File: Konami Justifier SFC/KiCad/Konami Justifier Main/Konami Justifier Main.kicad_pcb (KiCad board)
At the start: 4 copper layers, 25.2 x 50 mm, 19 parts, among them J1 RJ12, J2 Conn_01x06_Socket, U1 74VHC9164FT

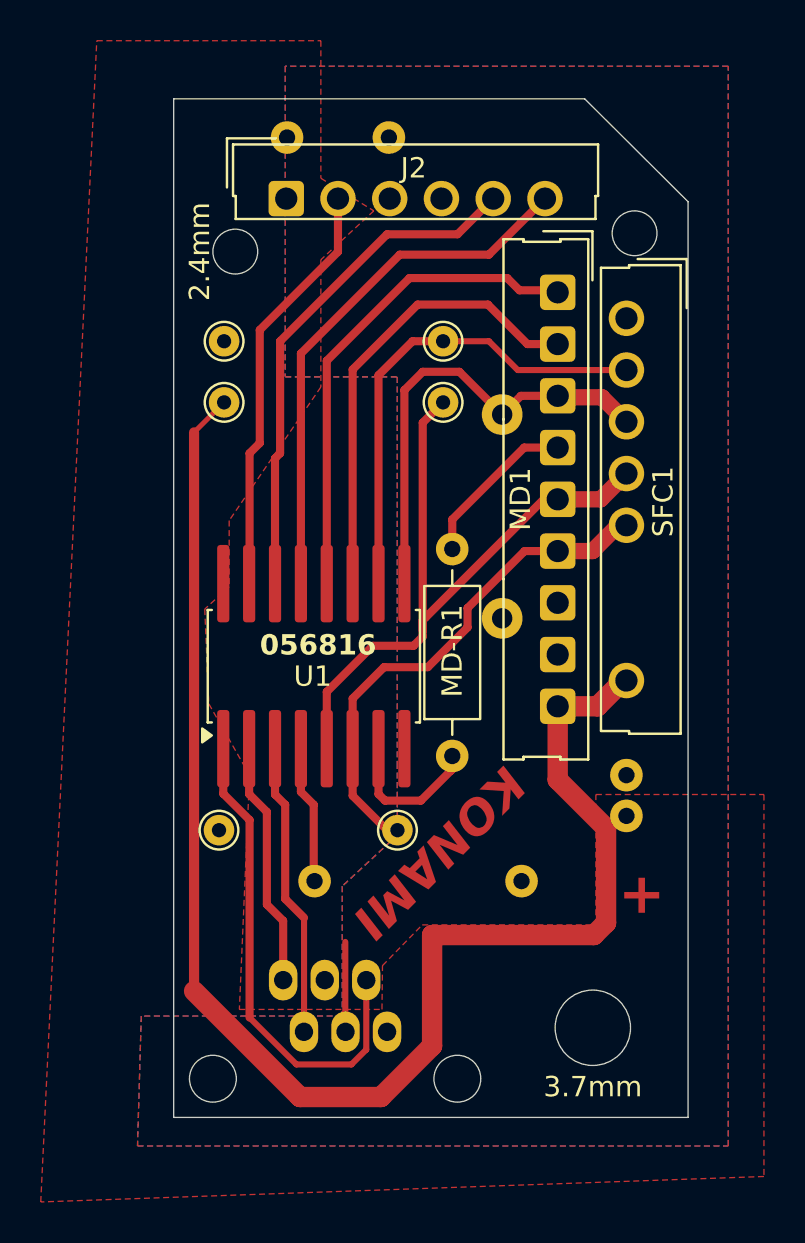
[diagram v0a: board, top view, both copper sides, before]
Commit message: Add files via upload
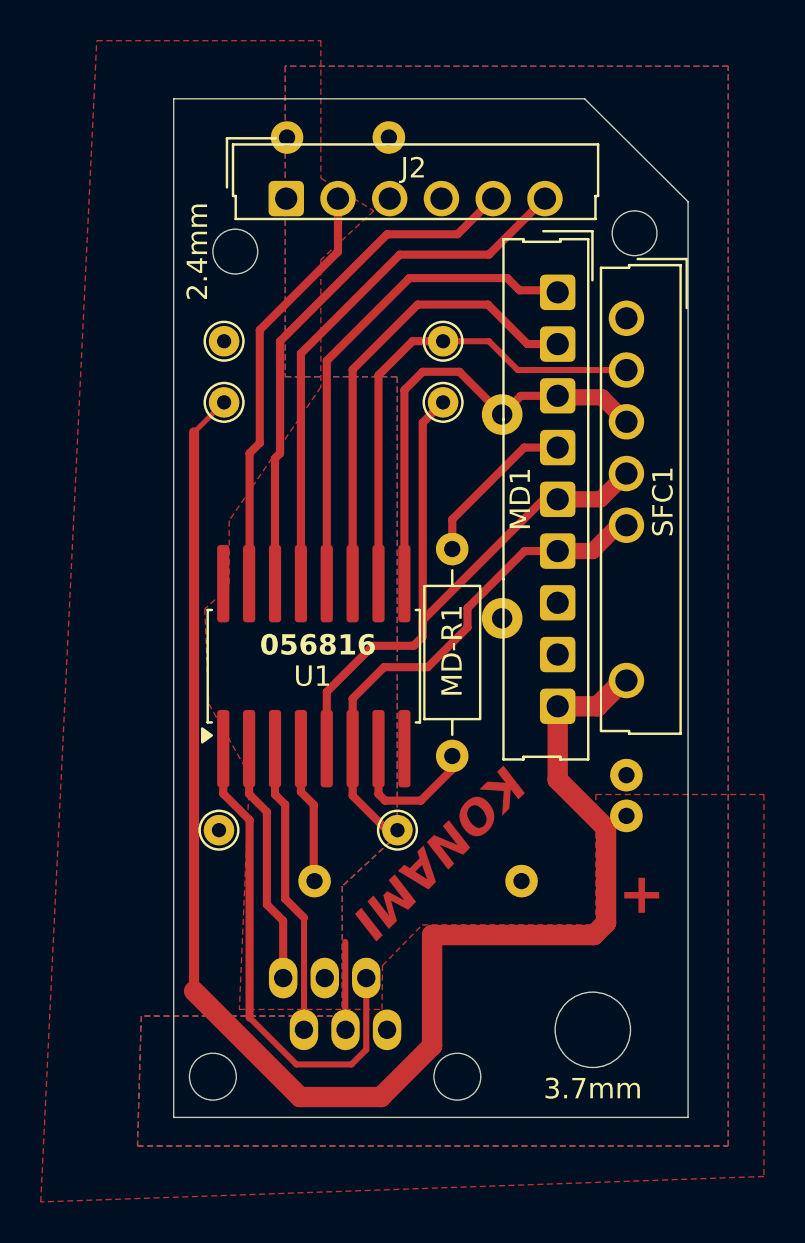
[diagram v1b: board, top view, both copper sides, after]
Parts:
- moved 3.7mm 0.10 mm to (160.3, 122.3)
- moved J1 0.10 mm to (145.2, 119.8)
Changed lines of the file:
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@@
 		(tags "mountinghole M2 DIN965")
 		(property "Reference" "2.4mm"
-			(at -1.75 0 90)
+			(at -1.85 0 90)
 			(layer "F.SilkS")
 			(effects
@@
 	(footprint "MountingHole:MountingHole_3.7mm"
 		(layer "F.Cu")
-		(at 160.35 122.2)
+		(at 160.35 122.3)
 		(descr "Mounting Hole 3.7mm, no annular, generated by kicad-footprint-generator mountinghole.py")
 		(tags "mountinghole")
@@
 	(footprint "Connector_RJ:RJ25_Wayconn_MJEA-660X1_Horizontal"
 		(layer "B.Cu")
-		(at 145.15 119.86 180)
+		(at 145.15 119.76 180)
 		(descr "RJ25 6P6C Socket 90 degrees, https://wayconn.com/wp-content/themes/way/datasheet/MJEA-660X1XXX_RJ25_6P6C_PCB_RA.pdf")
 		(tags "RJ12 RJ18 RJ25 jack connector 6P6C")
@@
 	)
 	(zone
-		(net 4)
-		(net_name "Net-(MD1-Pin_3)")
+		(net 13)
+		(net_name "Net-(MD1-Pin_5)")
 		(layer "F.Cu")
 		(name "$teardrop_padvia$")
 		(hatch none 0.1)
-		(priority 30003)
+		(priority 30001)
 		(attr
 			(teardrop
@@
 		(polygon
 			(pts
-				(xy 160.775843 90.85) (xy 160.775843 91.65) (xy 161.146717 92.624729) (xy 162.001 92.455) (xy 162.483346 91.731621)
+				(xy 160.498612 95.930703) (xy 161.064297 96.496388) (xy 162.483346 95.718379) (xy 162.000707 94.994293)
+				(xy 161.276621 94.511654)
 			)
 		)
 	)
 	(zone
-		(net 12)
-		(net_name "Net-(MD1-Pin_6)")
+		(net 6)
+		(net_name "+5V")
 		(layer "F.Cu")
 		(name "$teardrop_padvia$")
 		(hatch none 0.1)
-		(priority 30002)
+		(priority 30000)
 		(attr
 			(teardrop
@@
 		(polygon
 			(pts
-				(xy 160.331743 98.237572) (xy 160.897428 98.803257) (xy 162.169729 98.388283) (xy 162.000707 97.534293)
-				(xy 161.276621 97.051654)
+				(xy 160.350401 105.942492) (xy 161.057508 106.649599) (xy 162.483346 105.878379) (xy 162.000707 105.154293)
+				(xy 161.276621 104.671654)
 			)
 		)
 	)
 	(zone
-		(net 6)
-		(net_name "+5V")
+		(net 12)
+		(net_name "Net-(MD1-Pin_6)")
 		(layer "F.Cu")
 		(name "$teardrop_padvia$")
 		(hatch none 0.1)
-		(priority 30000)
+		(priority 30002)
 		(attr
 			(teardrop
@@
 		(polygon
 			(pts
-				(xy 160.350401 105.942492) (xy 161.057508 106.649599) (xy 162.483346 105.878379) (xy 162.000707 105.154293)
-				(xy 161.276621 104.671654)
+				(xy 160.331743 98.237572) (xy 160.897428 98.803257) (xy 162.169729 98.388283) (xy 162.000707 97.534293)
+				(xy 161.276621 97.051654)
 			)
 		)
 	)
 	(zone
-		(net 13)
-		(net_name "Net-(MD1-Pin_5)")
+		(net 4)
+		(net_name "Net-(MD1-Pin_3)")
 		(layer "F.Cu")
 		(name "$teardrop_padvia$")
 		(hatch none 0.1)
-		(priority 30001)
+		(priority 30003)
 		(attr
 			(teardrop
@@
 		(polygon
 			(pts
-				(xy 160.498612 95.930703) (xy 161.064297 96.496388) (xy 162.483346 95.718379) (xy 162.000707 94.994293)
-				(xy 161.276621 94.511654)
+				(xy 160.775843 90.85) (xy 160.775843 91.65) (xy 161.146717 92.624729) (xy 162.001 92.455) (xy 162.483346 91.731621)
 			)
 		)
